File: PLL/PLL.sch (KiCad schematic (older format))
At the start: 81 parts, among them J1 Clock, J10 Mix, J2 EuroPower, J3 D8, J4 D4, J5 D2, J6 M1, J7 M2, J8 M4, J9 M8, SW1 Lock speed, U1 TL082, U2 CD4046, U3 CD4040

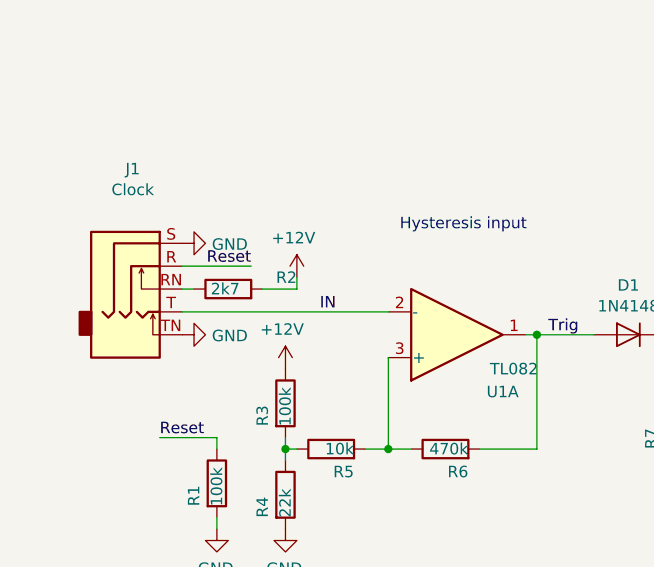
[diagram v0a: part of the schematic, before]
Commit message: PLL done
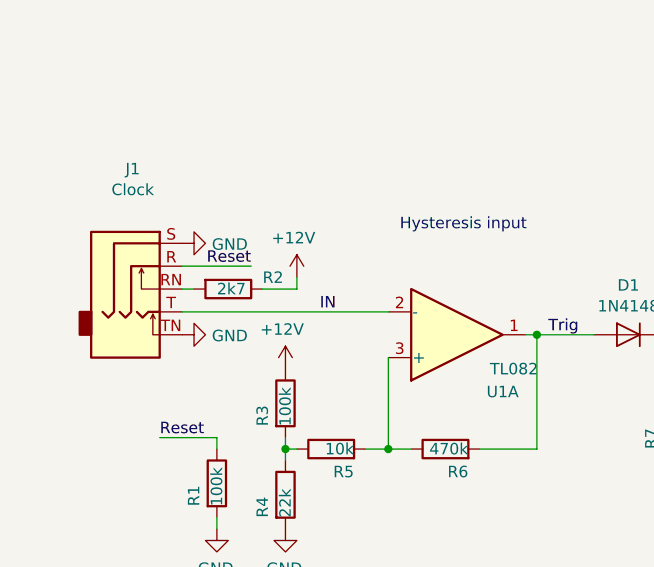
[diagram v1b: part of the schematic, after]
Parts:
- R1, R2: footprint Resistor_SMD:R_1206_3216Metric_Pad1.42x1.75mm_HandSolder -> Resistor_THT:R_Axial_DIN0204_L3.6mm_D1.6mm_P7.62mm_Horizontal
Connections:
- net +12V: now also R2.1; no longer R2.2
- net at J1.RN: now also R2.2; no longer R2.1
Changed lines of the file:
@@
-$EndComp
-$Comp
-L Device:R R2
-U 1 1 5F835D57
-P 1350 3200
-AR Path="/5F835D57" Ref="R2"  Part="1"
-AR Path="/5F42563C/5F835D57" Ref="R?"  Part="1"
-F 0 "R2" V 1400 2900 50  0000 L CNN
-F 1 "2k7" V 1350 3150 50  0000 L CNN
-F 2 "Resistor_SMD:R_1206_3216Metric_Pad1.42x1.75mm_HandSolder" V 1280 3200 50  0001 C CNN
-F 3 "~" H 1350 3200 50  0001 C CNN
-	1    1350 3200
-	0    -1   -1   0
 $EndComp
 $Comp
@@
 Wire Wire Line
 	1300 3850 1300 3900
-$Comp
-L Device:R R1
-U 1 1 5F89F815
-P 1300 4050
-AR Path="/5F89F815" Ref="R1"  Part="1"
-AR Path="/5F42563C/5F89F815" Ref="R?"  Part="1"
-AR Path="/5F425067/5F89F815" Ref="R?"  Part="1"
-F 0 "R1" V 1200 3950 50  0000 L CNN
-F 1 "100k" V 1300 3950 50  0000 L CNN
-F 2 "Resistor_SMD:R_1206_3216Metric_Pad1.42x1.75mm_HandSolder" V 1230 4050 50  0001 C CNN
-F 3 "~" H 1300 4050 50  0001 C CNN
-	1    1300 4050
-	1    0    0    -1
-$EndComp
 Wire Wire Line
 	1300 4250 1300 4200
@@
 	1    0    0    -1
 $EndComp
+$Comp
+L Device:R R1
+U 1 1 5F9EC571
+P 1300 4050
+AR Path="/5F9EC571" Ref="R1"  Part="1"
+AR Path="/5F42563C/5F9EC571" Ref="R?"  Part="1"
+AR Path="/5F425067/5F9EC571" Ref="R?"  Part="1"
+F 0 "R1" V 1200 3950 50  0000 L CNN
+F 1 "100k" V 1300 3950 50  0000 L CNN
+F 2 "Resistor_THT:R_Axial_DIN0204_L3.6mm_D1.6mm_P7.62mm_Horizontal" V 1230 4050 50  0001 C CNN
+F 3 "~" H 1300 4050 50  0001 C CNN
+	1    1300 4050
+	1    0    0    -1
+$EndComp
+$Comp
+L Device:R R2
+U 1 1 5F9EDF49
+P 1350 3200
+AR Path="/5F9EDF49" Ref="R2"  Part="1"
+AR Path="/5F42563C/5F9EDF49" Ref="R?"  Part="1"
+AR Path="/5F425067/5F9EDF49" Ref="R?"  Part="1"
+F 0 "R2" V 1300 3350 50  0000 L CNN
+F 1 "2k7" V 1350 3150 50  0000 L CNN
+F 2 "Resistor_THT:R_Axial_DIN0204_L3.6mm_D1.6mm_P7.62mm_Horizontal" V 1280 3200 50  0001 C CNN
+F 3 "~" H 1350 3200 50  0001 C CNN
+	1    1350 3200
+	0    1    1    0
+$EndComp
 $EndSCHEMATC
